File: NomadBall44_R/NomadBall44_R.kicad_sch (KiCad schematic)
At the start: 52 parts, among them SW1 SW_Push, SW10 SW_Push, SW11 SW_Push, SW12 SW_Push, SW13 SW_Push, SW14 SW_Push, SW15 SW_Push, SW16 SW_Push, SW17 SW_Push, SW18 SW_Push, SW19 SW_Push, SW2 SW_Push, SW20 SW_Push, SW21 SW_Push, SW22 SW_Push, SW23 SW_Push, SW25 SW_SPDT, SW26 RotaryEncoder_Switch, SW3 SW_Push, SW4 SW_Push, SW5 SW_Push, SW6 SW_Push, SW7 SW_Push, SW8 SW_Push, SW9 SW_Push, U1 XIAO-nRF52840-Plus-SMD

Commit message: ロータリエンコーダーのフットプリントを割り当て
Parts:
- SW26: footprint (none) -> Rotary_Encoder:RotaryEncoder_Alps_EC12E-Switch_Vertical_H20mm
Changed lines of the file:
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@@
 			)
 		)
-		(property "Footprint" ""
+		(property "Footprint" "Rotary_Encoder:RotaryEncoder_Alps_EC12E-Switch_Vertical_H20mm"
 			(at 138.43 107.696 0)
 			(effects

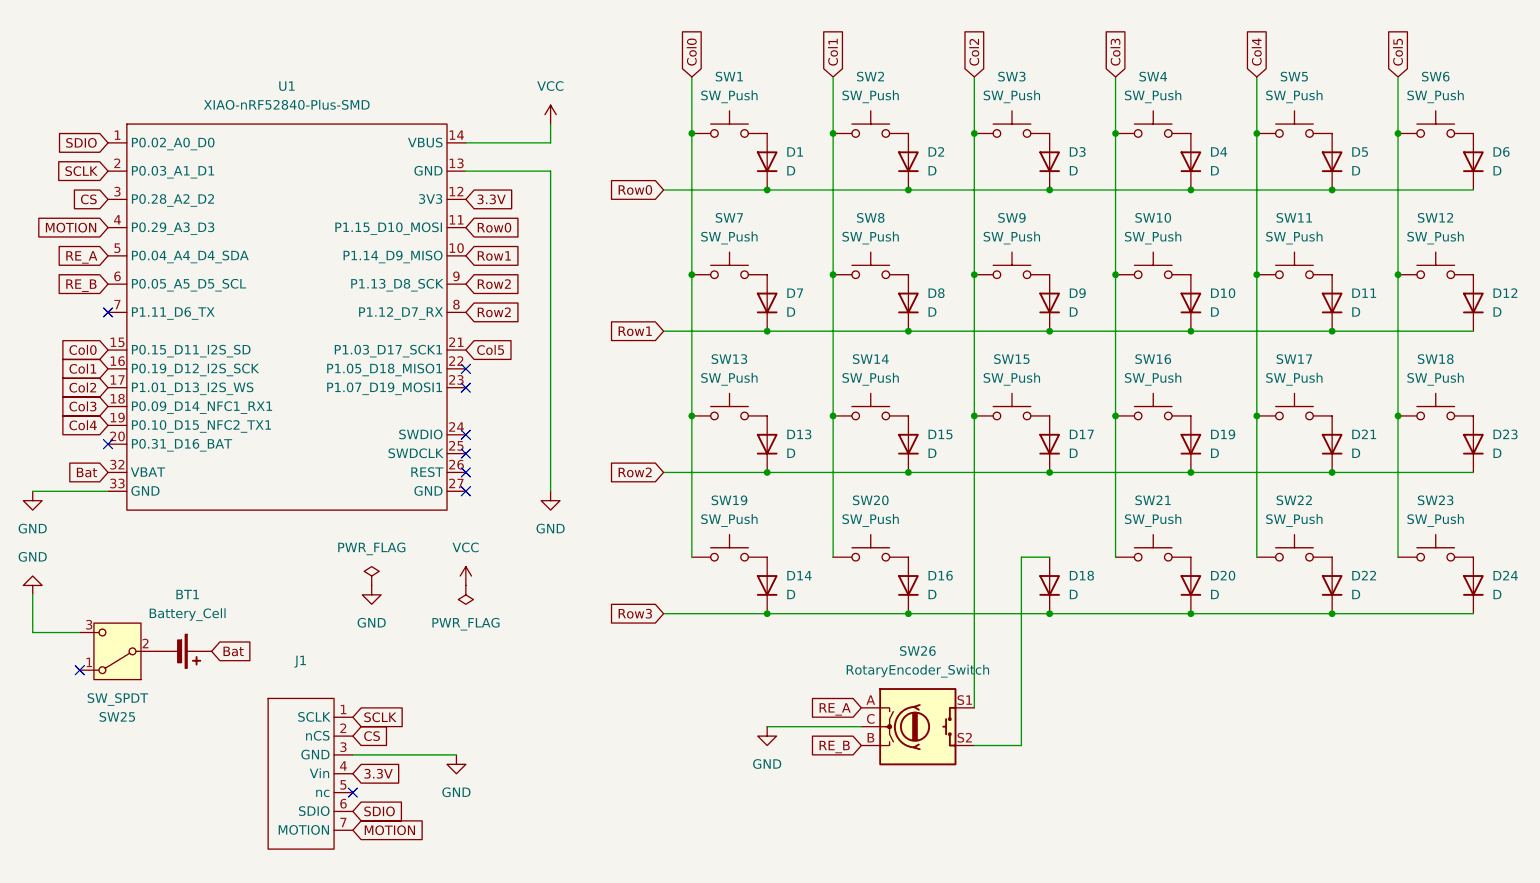
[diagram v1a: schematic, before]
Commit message: NomadBall44用のシンボルライブラリを作成
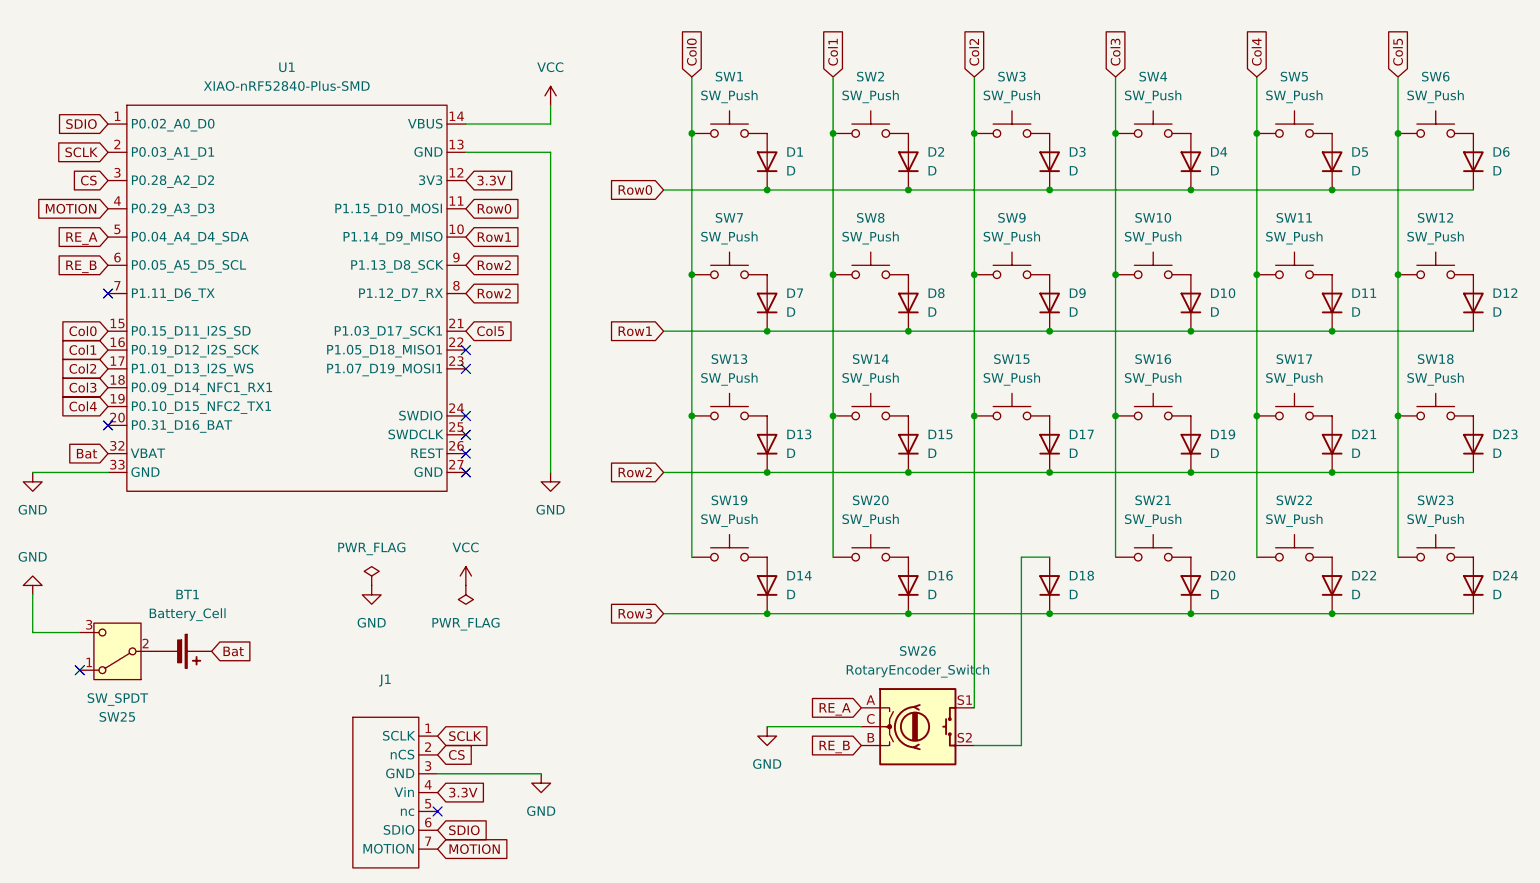
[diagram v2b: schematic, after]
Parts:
- removed J1: ~, myfootprintLibrary:pmw3610_connector, symbol roba:pmw3610_breakout
- removed U1: XIAO-nRF52840-Plus-SMD, footprints:XIAO-nRF52840-Plus-Through-Hole, symbol Seeed_Studio_XIAO_Series:XIAO-nRF52840_Plus_SMD
- added J1: ~, myfootprintLibrary:pmw3610_connector, symbol NomadBall44:pmw3610_breakout
- added U1: XIAO-nRF52840-Plus-SMD, footprints:XIAO-nRF52840-Plus, symbol NomadBall44:XIAO-nRF52840_Plus_SMD
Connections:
- net 3.3V: now also J1.4 (Vin), U1.12 (3V3)
- net Bat: now also U1.32 (VBAT)
- net CS: now also J1.2 (nCS), U1.3 (P0.28_A2_D2)
- net Col0: now also U1.15 (P0.15_D11_I2S_SD)
- net Col1: now also U1.16 (P0.19_D12_I2S_SCK)
- net Col2: now also U1.17 (P1.01_D13_I2S_WS)
- net Col3: now also U1.18 (P0.09_D14_NFC1_RX1)
- net Col4: now also U1.19 (P0.10_D15_NFC2_TX1)
- net Col5: now also U1.21 (P1.03_D17_SCK1)
- net GND: now also J1.3 (GND), U1.13 (GND), U1.33 (GND)
- net MOTION: now also J1.7 (MOTION), U1.4 (P0.29_A3_D3)
- net RE_A: now also U1.5 (P0.04_A4_D4_SDA)
- net RE_B: now also U1.6 (P0.05_A5_D5_SCL)
- net Row0: now also U1.11 (P1.15_D10_MOSI)
- net Row1: now also U1.10 (P1.14_D9_MISO)
- net Row2: now also U1.8 (P1.12_D7_RX), U1.9 (P1.13_D8_SCK)
- net SCLK: now also J1.1 (SCLK), U1.2 (P0.03_A1_D1)
- net SDIO: now also J1.6 (SDIO), U1.1 (P0.02_A0_D0)
- net VCC: now also U1.14 (VBUS)
